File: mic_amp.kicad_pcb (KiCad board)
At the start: 2 copper layers, 41.4 x 28.6 mm, 24 parts

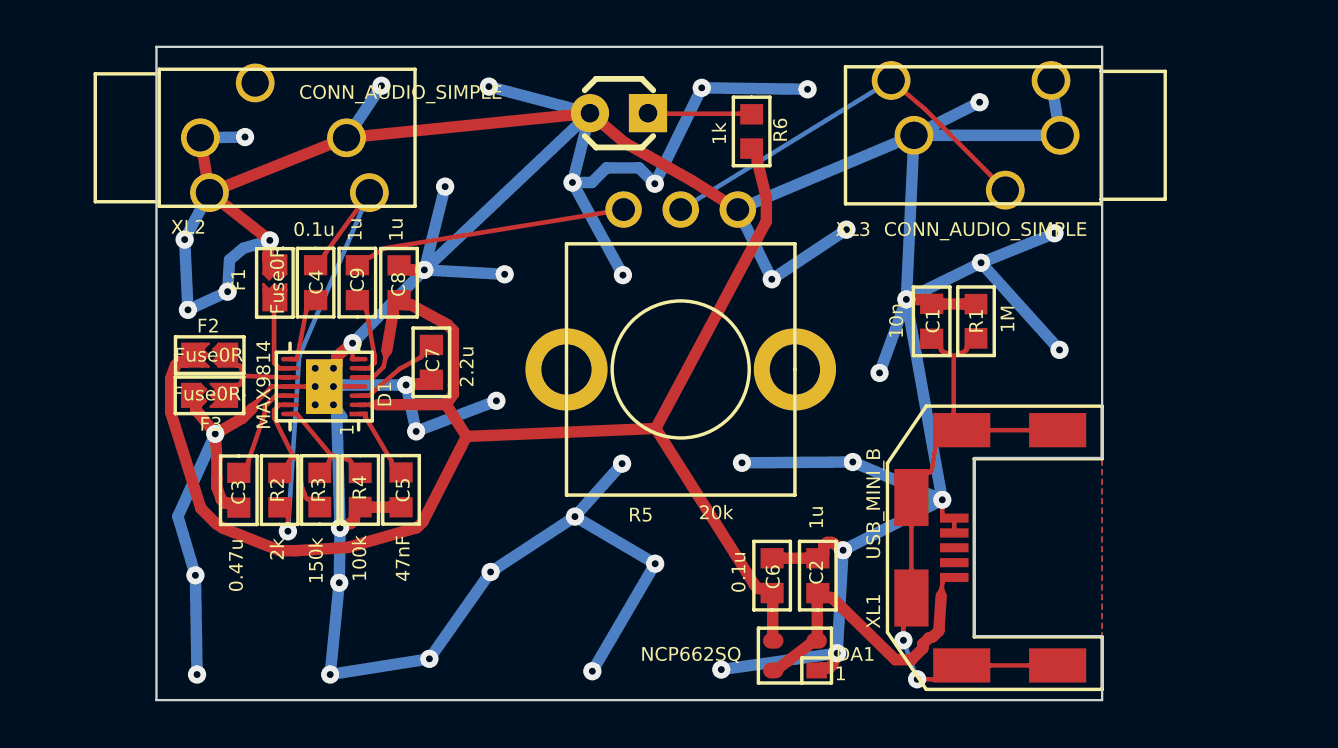
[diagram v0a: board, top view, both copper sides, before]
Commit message: With 3v battery
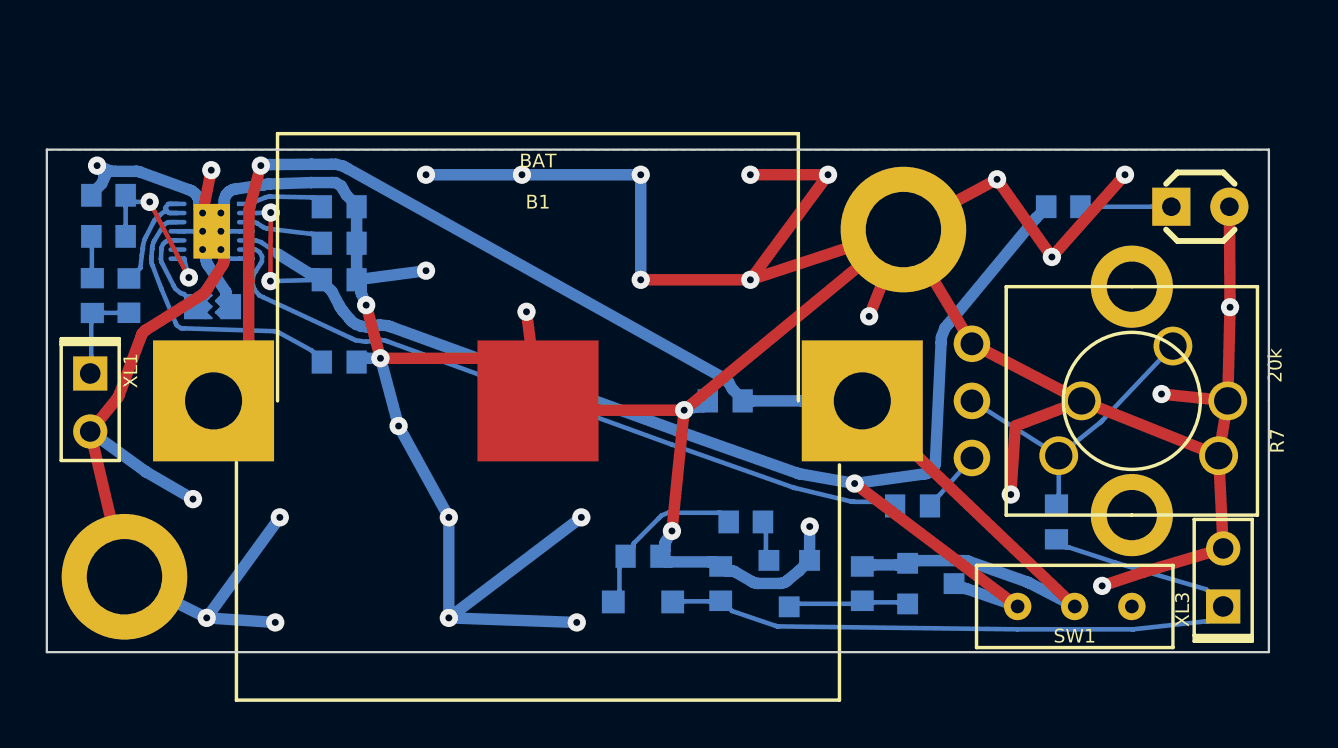
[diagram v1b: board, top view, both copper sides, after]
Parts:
- removed the C1 at (223.7, 100.4)
- removed the C2 at (218.8, 111.6)
- removed the D1 at (197.1, 103.3)
- removed DA1: NCP662SQ, SOT:SC82AB
- removed the F1 at (195.0, 98.7)
- removed F2: Fuse0R, Resistors:RES_0603_SOLDERFUSE
- removed the R1 at (225.7, 100.4)
- removed the XL2 at (189.9, 92.4)
- added B1: BAT, Installation:BAT_HOLDER_BHX1-2032-SM, F.Cu at (206.5, 103.9)
- added C8: 1u, Capacitors:CAP_0603, B.Cu at (211.1, 110.7)
- added C9: 1u, Capacitors:CAP_0603, B.Cu at (229.2, 109.2)
- added D2: MAX9814, QFN_DFN:DFN14, B.Cu at (192.2, 96.5)
- added D3: BAT54WS, Diodes:SOD323, B.Cu at (211.1, 112.7)
- added HOLE1: HOLE_METALLED, PCB:Hole3d3_out5d5mm, F.Cu at (188.4, 111.6)
- added HOLE2: HOLE_METALLED, PCB:Hole3d3_out5d5mm, F.Cu at (222.5, 96.4)
- added Q1: IRLML9303, SOT:SOT23-3, B.Cu at (223.7, 111.9)
- added Q2: BC848, SOT:SOT23-3, B.Cu at (217.5, 111.9)
- added R2: 0R, Resistors:RES_0603, B.Cu at (187.7, 96.7)
- added R5: 20k, Resistors:RES_0603, B.Cu at (220.7, 111.9)
- added R8: 2k, Resistors:RES_0603, B.Cu at (214.5, 111.9)
- added SW1: SWITCH, BtnsSwitches:SW_SS-1P2T, F.Cu at (230.0, 112.9)
- added XL3: CONN_2, Connectors:PLS-2, F.Cu at (236.5, 112.9)
- C1: renamed from C4; moved to B.Cu
- C2: renamed from C3; moved to B.Cu
- C3: renamed from C5; moved to B.Cu
- C4: renamed from C7; moved to B.Cu
- C5: renamed from C6; value 0.1u -> 10u; moved to B.Cu
- C6: renamed from C8; value 1u -> 0.1u; moved to B.Cu
- C7: renamed from C9; moved to B.Cu
- F1: renamed from F3; moved to B.Cu
- R1: renamed from R2; moved to B.Cu
- R3: value 150k -> DNM; moved to B.Cu
- R4: value 100k -> 2k; moved to B.Cu
- R6: value 1k -> 2k; moved to B.Cu
- XL1: value USB_MINI_B -> CONN_2; footprint Connectors:USBmicro_MOLEX_WM17142 -> Connectors:PLS-2
- XL2: renamed from XL3; moved to B.Cu
- moved XL1 39.4 mm to (186.9, 102.7), turned to 270 degrees
- moved R4 33.2 mm to (229.5, 95.4), turned to 0 degrees
- moved C7 26.2 mm to (222.9, 108.5), turned to 0 degrees
- moved D1 25.8 mm to (235.5, 95.4), turned to 0 degrees
- moved R7 19.8 mm to (232.5, 103.9), turned to 270 degrees
- moved R6 17.1 mm to (215.6, 109.2), turned to 180 degrees
- moved R3 15.9 mm to (187.7, 94.9), turned to 180 degrees
- moved XL2 13.7 mm to (238.5, 103.9)
- moved C3 12.7 mm to (197.8, 95.4), turned to 0 degrees
- moved R1 10.8 mm to (188.6, 99.3)
- moved C1 9.79 mm to (187.0, 99.3), turned to 90 degrees
- moved C5 7.92 mm to (214.7, 103.9), turned to 180 degrees
- moved C2 7.13 mm to (197.8, 102.2), turned to 0 degrees
- moved C4 6.59 mm to (197.8, 97.0), turned to 0 degrees
- moved F1 3.88 mm to (192.3, 99.8), turned to 0 degrees
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- renumbered D2 to D1, R5 to R7
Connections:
- C1 pad 1: Net-(C4-Pad1) (its old number) -> Net-(C1-Pad1)
- C1 pad 2: /MICIN -> Net-(C1-Pad2)
- C5 pad 1: VDD -> /BAT_IN
- D1 pad A: Net-(D2-PadA) -> Net-(D1-PadA)
- R1 pad 1: Net-(C4-Pad1) (its old number) -> Net-(C1-Pad1)
- R3 pad 1: /MICBIAS -> /MICIN
- R3 pad 2: Net-(D1-Pad14) -> GND
- R4 pad 1: Net-(D1-Pad14) -> VDD
- R4 pad 2: GND -> Net-(D1-PadA)
- R6 pad 1: Net-(D2-PadA) -> Net-(Q2-Pad1)
- R6 pad 2: VDD -> Net-(C8-Pad1)
- XL1 pad 1: Net-(C2-Pad1) (its old number) -> Net-(C1-Pad1)
- XL1 pad 2: Net-(XL1-Pad2) -> GND
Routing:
- net /BAT_IN: track 0.00 -> 62.8 mm, vias 0 -> 1
- net Net-(C9-Pad2): track 0.00 -> 32.7 mm
- net GND: track 267.1 -> 234.8 mm, vias 45 -> 32
- net Net-(C7-Pad1): track 3.77 -> 32.3 mm
- net Net-(C1-Pad1): track 28.6 -> 4.25 mm, vias 2 -> 0
- net Net-(C4-Pad1) (its old number): track 20.7 -> 0.00 mm, vias 1 -> 0
- net Net-(C2-Pad1) (its old number): track 15.0 -> 0.00 mm
- net Net-(C7-Pad2): track 12.0 -> 2.79 mm
- net Net-(C8-Pad1): track 0.00 -> 7.72 mm
- net Net-(C2-Pad1): track 4.52 -> 12.2 mm
- net VDD: track 72.4 -> 65.0 mm, vias 0 -> 3
- net (no net): track 0.00 -> 5.38 mm, vias 0 -> 1
- net Net-(Q1-Pad1): track 0.00 -> 5.24 mm
- net Net-(D1-Pad14): track 5.21 -> 0.00 mm
- net /MICIN: track 3.12 -> 7.83 mm, vias 0 -> 2
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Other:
- board size 41.4 x 28.6 mm -> 53.5 x 22 mm
- board text added: "F1: Soldered => 50dB Not soldered => 60dB"
- board text added: "StetoAmp 2"
